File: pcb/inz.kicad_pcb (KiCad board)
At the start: 2 copper layers, 410 parts, among them U1 AMS1117-3.3, U2 ESP32-S3-WROOM-1

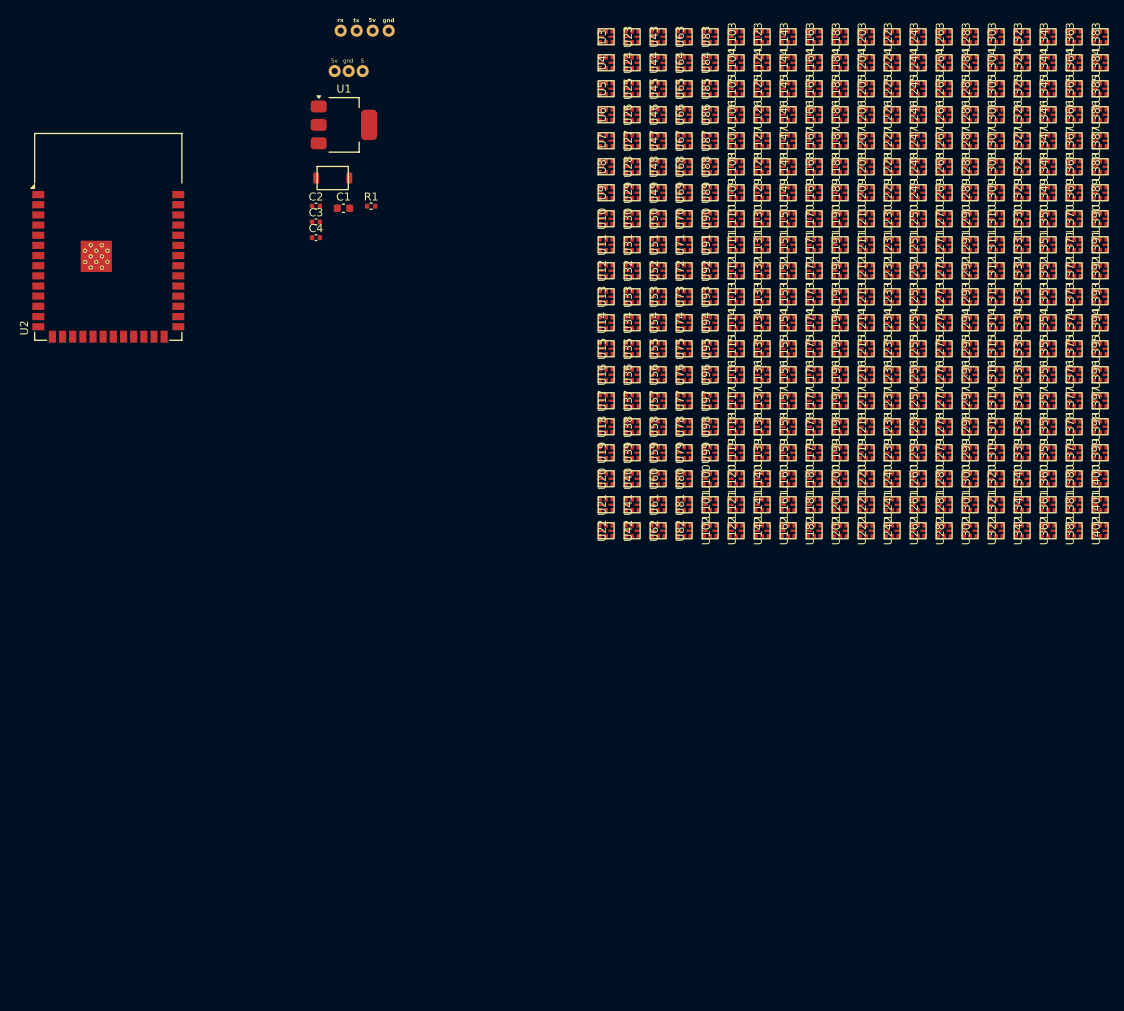
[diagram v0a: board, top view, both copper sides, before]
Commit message: pcb update
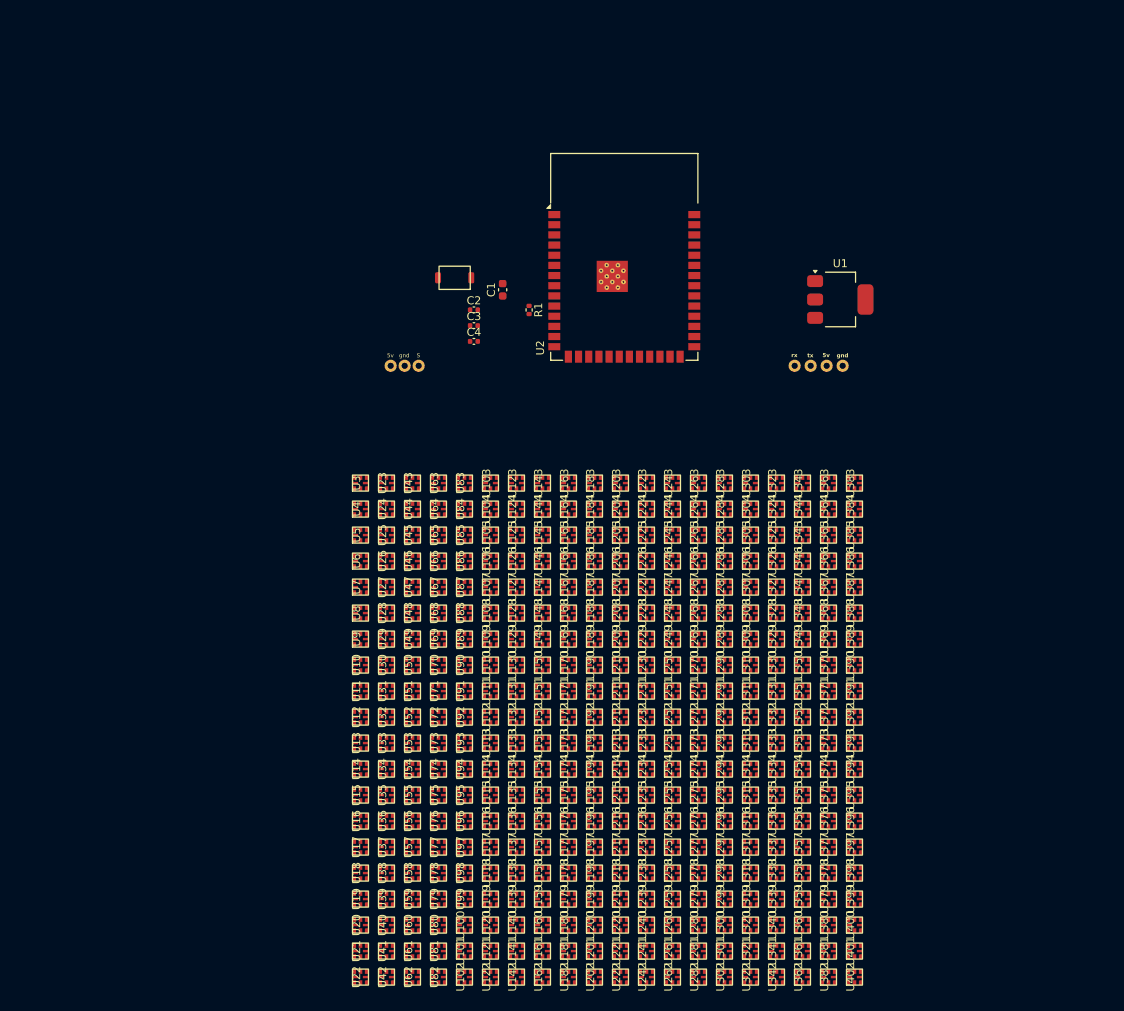
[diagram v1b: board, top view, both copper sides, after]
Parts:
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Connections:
- U103 pad 3: Net-(U103-CLI) -> Net-(U102-CLO)
- U103 pad 6: Net-(U103-DAI) -> Net-(U102-DAO)
- U104 pad 1: Net-(U103-CLI) -> Net-(U104-CLO)
- U104 pad 3: Net-(U104-CLI) -> Net-(U103-CLO)
- U104 pad 4: Net-(U103-DAI) -> Net-(U104-DAO)
- U104 pad 6: Net-(U104-DAI) -> Net-(U103-DAO)
- U105 pad 1: Net-(U104-CLI) -> Net-(U105-CLO)
- U105 pad 3: Net-(U105-CLI) -> Net-(U104-CLO)
- U105 pad 4: Net-(U104-DAI) -> Net-(U105-DAO)
- U105 pad 6: Net-(U105-DAI) -> Net-(U104-DAO)
- U106 pad 1: Net-(U105-CLI) -> Net-(U106-CLO)
- U106 pad 3: Net-(U106-CLI) -> Net-(U105-CLO)
- U106 pad 4: Net-(U105-DAI) -> Net-(U106-DAO)
- U106 pad 6: Net-(U106-DAI) -> Net-(U105-DAO)
- U107 pad 1: Net-(U106-CLI) -> Net-(U107-CLO)
- U107 pad 3: Net-(U107-CLI) -> Net-(U106-CLO)
- U107 pad 4: Net-(U106-DAI) -> Net-(U107-DAO)
- U107 pad 6: Net-(U107-DAI) -> Net-(U106-DAO)
- U108 pad 1: Net-(U107-CLI) -> Net-(U108-CLO)
- U108 pad 3: Net-(U108-CLI) -> Net-(U107-CLO)
- U108 pad 4: Net-(U107-DAI) -> Net-(U108-DAO)
- U108 pad 6: Net-(U108-DAI) -> Net-(U107-DAO)
- U109 pad 1: Net-(U108-CLI) -> Net-(U109-CLO)
- U109 pad 3: Net-(U109-CLI) -> Net-(U108-CLO)
- U109 pad 4: Net-(U108-DAI) -> Net-(U109-DAO)
- U109 pad 6: Net-(U109-DAI) -> Net-(U108-DAO)
- U110 pad 1: Net-(U109-CLI) -> Net-(U110-CLO)
- U110 pad 3: Net-(U110-CLI) -> Net-(U109-CLO)
- U110 pad 4: Net-(U109-DAI) -> Net-(U110-DAO)
- U110 pad 6: Net-(U110-DAI) -> Net-(U109-DAO)
- U111 pad 1: Net-(U110-CLI) -> Net-(U111-CLO)
- U111 pad 3: Net-(U111-CLI) -> Net-(U110-CLO)
- U111 pad 4: Net-(U110-DAI) -> Net-(U111-DAO)
- U111 pad 6: Net-(U111-DAI) -> Net-(U110-DAO)
- U112 pad 1: Net-(U111-CLI) -> Net-(U112-CLO)
- U112 pad 3: Net-(U112-CLI) -> Net-(U111-CLO)
- U112 pad 4: Net-(U111-DAI) -> Net-(U112-DAO)
- U112 pad 6: Net-(U112-DAI) -> Net-(U111-DAO)
- U113 pad 1: Net-(U112-CLI) -> Net-(U113-CLO)
- U113 pad 3: Net-(U113-CLI) -> Net-(U112-CLO)
- U113 pad 4: Net-(U112-DAI) -> Net-(U113-DAO)
- U113 pad 6: Net-(U113-DAI) -> Net-(U112-DAO)
- U114 pad 1: Net-(U113-CLI) -> Net-(U114-CLO)
- U114 pad 3: Net-(U114-CLI) -> Net-(U113-CLO)
- U114 pad 4: Net-(U113-DAI) -> Net-(U114-DAO)
- U114 pad 6: Net-(U114-DAI) -> Net-(U113-DAO)
- U115 pad 1: Net-(U114-CLI) -> Net-(U115-CLO)
- U115 pad 3: Net-(U115-CLI) -> Net-(U114-CLO)
- U115 pad 4: Net-(U114-DAI) -> Net-(U115-DAO)
- U115 pad 6: Net-(U115-DAI) -> Net-(U114-DAO)
- U116 pad 1: Net-(U115-CLI) -> Net-(U116-CLO)
- U116 pad 3: Net-(U116-CLI) -> Net-(U115-CLO)
- U116 pad 4: Net-(U115-DAI) -> Net-(U116-DAO)
- U116 pad 6: Net-(U116-DAI) -> Net-(U115-DAO)
- U117 pad 1: Net-(U116-CLI) -> Net-(U117-CLO)
- U117 pad 3: Net-(U117-CLI) -> Net-(U116-CLO)
- U117 pad 4: Net-(U116-DAI) -> Net-(U117-DAO)
- U117 pad 6: Net-(U117-DAI) -> Net-(U116-DAO)
- U118 pad 1: Net-(U117-CLI) -> Net-(U118-CLO)
- U118 pad 3: Net-(U118-CLI) -> Net-(U117-CLO)
- U118 pad 4: Net-(U117-DAI) -> Net-(U118-DAO)
- U118 pad 6: Net-(U118-DAI) -> Net-(U117-DAO)
- U119 pad 1: Net-(U118-CLI) -> Net-(U119-CLO)
- U119 pad 3: Net-(U119-CLI) -> Net-(U118-CLO)
- U119 pad 4: Net-(U118-DAI) -> Net-(U119-DAO)
- U119 pad 6: Net-(U119-DAI) -> Net-(U118-DAO)
- U120 pad 1: Net-(U119-CLI) -> Net-(U120-CLO)
- U120 pad 3: Net-(U120-CLI) -> Net-(U119-CLO)
- U120 pad 4: Net-(U119-DAI) -> Net-(U120-DAO)
- U120 pad 6: Net-(U120-DAI) -> Net-(U119-DAO)
- U121 pad 1: Net-(U120-CLI) -> Net-(U121-CLO)
- U121 pad 3: Net-(U121-CLI) -> Net-(U120-CLO)
- U121 pad 4: Net-(U120-DAI) -> Net-(U121-DAO)
- U121 pad 6: Net-(U121-DAI) -> Net-(U120-DAO)
- U122 pad 1: Net-(U121-CLI) -> Net-(U122-CLO)
- U122 pad 3: Net-(U102-CLO) -> Net-(U121-CLO)
- U122 pad 4: Net-(U121-DAI) -> Net-(U122-DAO)
- U122 pad 6: Net-(U102-DAO) -> Net-(U121-DAO)
- U123 pad 3: Net-(U103-CLO) -> Net-(U122-CLO)
- U123 pad 6: Net-(U103-DAO) -> Net-(U122-DAO)
- U143 pad 3: Net-(U143-CLI) -> Net-(U142-CLO)
- U143 pad 6: Net-(U143-DAI) -> Net-(U142-DAO)
- U144 pad 1: Net-(U143-CLI) -> Net-(U144-CLO)
- U144 pad 3: Net-(U144-CLI) -> Net-(U143-CLO)
- U144 pad 4: Net-(U143-DAI) -> Net-(U144-DAO)
- U144 pad 6: Net-(U144-DAI) -> Net-(U143-DAO)
- U145 pad 1: Net-(U144-CLI) -> Net-(U145-CLO)
- U145 pad 3: Net-(U145-CLI) -> Net-(U144-CLO)
- U145 pad 4: Net-(U144-DAI) -> Net-(U145-DAO)
- U145 pad 6: Net-(U145-DAI) -> Net-(U144-DAO)
- U146 pad 1: Net-(U145-CLI) -> Net-(U146-CLO)
- U146 pad 3: Net-(U146-CLI) -> Net-(U145-CLO)
- U146 pad 4: Net-(U145-DAI) -> Net-(U146-DAO)
- U146 pad 6: Net-(U146-DAI) -> Net-(U145-DAO)
- U147 pad 1: Net-(U146-CLI) -> Net-(U147-CLO)
- U147 pad 3: Net-(U147-CLI) -> Net-(U146-CLO)
- U147 pad 4: Net-(U146-DAI) -> Net-(U147-DAO)
- U147 pad 6: Net-(U147-DAI) -> Net-(U146-DAO)
- U148 pad 1: Net-(U147-CLI) -> Net-(U148-CLO)
- U148 pad 3: Net-(U148-CLI) -> Net-(U147-CLO)
- U148 pad 4: Net-(U147-DAI) -> Net-(U148-DAO)
- U148 pad 6: Net-(U148-DAI) -> Net-(U147-DAO)
- U149 pad 1: Net-(U148-CLI) -> Net-(U149-CLO)
- U149 pad 3: Net-(U149-CLI) -> Net-(U148-CLO)
- U149 pad 4: Net-(U148-DAI) -> Net-(U149-DAO)
- U149 pad 6: Net-(U149-DAI) -> Net-(U148-DAO)
- U150 pad 1: Net-(U149-CLI) -> Net-(U150-CLO)
- U150 pad 3: Net-(U150-CLI) -> Net-(U149-CLO)
- U150 pad 4: Net-(U149-DAI) -> Net-(U150-DAO)
- U150 pad 6: Net-(U150-DAI) -> Net-(U149-DAO)
- U151 pad 1: Net-(U150-CLI) -> Net-(U151-CLO)
- U151 pad 3: Net-(U151-CLI) -> Net-(U150-CLO)
- U151 pad 4: Net-(U150-DAI) -> Net-(U151-DAO)
- U151 pad 6: Net-(U151-DAI) -> Net-(U150-DAO)
- U152 pad 1: Net-(U151-CLI) -> Net-(U152-CLO)
- U152 pad 3: Net-(U152-CLI) -> Net-(U151-CLO)
- U152 pad 4: Net-(U151-DAI) -> Net-(U152-DAO)
- U152 pad 6: Net-(U152-DAI) -> Net-(U151-DAO)
- U153 pad 1: Net-(U152-CLI) -> Net-(U153-CLO)
- U153 pad 3: Net-(U153-CLI) -> Net-(U152-CLO)
- U153 pad 4: Net-(U152-DAI) -> Net-(U153-DAO)
- U153 pad 6: Net-(U153-DAI) -> Net-(U152-DAO)
- U154 pad 1: Net-(U153-CLI) -> Net-(U154-CLO)
- U154 pad 3: Net-(U154-CLI) -> Net-(U153-CLO)
- U154 pad 4: Net-(U153-DAI) -> Net-(U154-DAO)
- U154 pad 6: Net-(U154-DAI) -> Net-(U153-DAO)
- U155 pad 1: Net-(U154-CLI) -> Net-(U155-CLO)
- U155 pad 3: Net-(U155-CLI) -> Net-(U154-CLO)
- U155 pad 4: Net-(U154-DAI) -> Net-(U155-DAO)
- U155 pad 6: Net-(U155-DAI) -> Net-(U154-DAO)
- U156 pad 1: Net-(U155-CLI) -> Net-(U156-CLO)
- U156 pad 3: Net-(U156-CLI) -> Net-(U155-CLO)
- U156 pad 4: Net-(U155-DAI) -> Net-(U156-DAO)
- U156 pad 6: Net-(U156-DAI) -> Net-(U155-DAO)
- U157 pad 1: Net-(U156-CLI) -> Net-(U157-CLO)
- U157 pad 3: Net-(U157-CLI) -> Net-(U156-CLO)
- U157 pad 4: Net-(U156-DAI) -> Net-(U157-DAO)
- U157 pad 6: Net-(U157-DAI) -> Net-(U156-DAO)
- U158 pad 1: Net-(U157-CLI) -> Net-(U158-CLO)
- U158 pad 3: Net-(U158-CLI) -> Net-(U157-CLO)
- U158 pad 4: Net-(U157-DAI) -> Net-(U158-DAO)
- U158 pad 6: Net-(U158-DAI) -> Net-(U157-DAO)
- U159 pad 1: Net-(U158-CLI) -> Net-(U159-CLO)
- U159 pad 3: Net-(U159-CLI) -> Net-(U158-CLO)
- U159 pad 4: Net-(U158-DAI) -> Net-(U159-DAO)
- U159 pad 6: Net-(U159-DAI) -> Net-(U158-DAO)
- U160 pad 1: Net-(U159-CLI) -> Net-(U160-CLO)
- U160 pad 3: Net-(U160-CLI) -> Net-(U159-CLO)
- U160 pad 4: Net-(U159-DAI) -> Net-(U160-DAO)
- U160 pad 6: Net-(U160-DAI) -> Net-(U159-DAO)
- U161 pad 1: Net-(U160-CLI) -> Net-(U161-CLO)
- U161 pad 3: Net-(U161-CLI) -> Net-(U160-CLO)
- U161 pad 4: Net-(U160-DAI) -> Net-(U161-DAO)
- U161 pad 6: Net-(U161-DAI) -> Net-(U160-DAO)
- U162 pad 1: Net-(U161-CLI) -> Net-(U162-CLO)
- U162 pad 3: Net-(U142-CLO) -> Net-(U161-CLO)
- U162 pad 4: Net-(U161-DAI) -> Net-(U162-DAO)
- U162 pad 6: Net-(U142-DAO) -> Net-(U161-DAO)
- U163 pad 3: Net-(U143-CLO) -> Net-(U162-CLO)
- U163 pad 6: Net-(U143-DAO) -> Net-(U162-DAO)
- U183 pad 1: unconnected-(U183-CLO-Pad1) -> Net-(U183-CLO)
- U183 pad 3: Net-(U183-CLI) -> Net-(U182-CLO)
- U183 pad 4: unconnected-(U183-DAO-Pad4) -> Net-(U183-DAO)
- U183 pad 6: Net-(U183-DAI) -> Net-(U182-DAO)
- U184 pad 1: Net-(U183-CLI) -> Net-(U184-CLO)
- U184 pad 3: Net-(U184-CLI) -> Net-(U183-CLO)
- U184 pad 4: Net-(U183-DAI) -> Net-(U184-DAO)
- U184 pad 6: Net-(U184-DAI) -> Net-(U183-DAO)
- U185 pad 1: Net-(U184-CLI) -> Net-(U185-CLO)
- U185 pad 3: Net-(U185-CLI) -> Net-(U184-CLO)
- U185 pad 4: Net-(U184-DAI) -> Net-(U185-DAO)
- U185 pad 6: Net-(U185-DAI) -> Net-(U184-DAO)
- U186 pad 1: Net-(U185-CLI) -> Net-(U186-CLO)
- U186 pad 3: Net-(U186-CLI) -> Net-(U185-CLO)
- U186 pad 4: Net-(U185-DAI) -> Net-(U186-DAO)
- U186 pad 6: Net-(U186-DAI) -> Net-(U185-DAO)
- U187 pad 1: Net-(U186-CLI) -> Net-(U187-CLO)
- U187 pad 3: Net-(U187-CLI) -> Net-(U186-CLO)
- U187 pad 4: Net-(U186-DAI) -> Net-(U187-DAO)
- U187 pad 6: Net-(U187-DAI) -> Net-(U186-DAO)
- U188 pad 1: Net-(U187-CLI) -> Net-(U188-CLO)
- U188 pad 3: Net-(U188-CLI) -> Net-(U187-CLO)
- U188 pad 4: Net-(U187-DAI) -> Net-(U188-DAO)
- U188 pad 6: Net-(U188-DAI) -> Net-(U187-DAO)
- U189 pad 1: Net-(U188-CLI) -> Net-(U189-CLO)
- U189 pad 3: Net-(U189-CLI) -> Net-(U188-CLO)
- U189 pad 4: Net-(U188-DAI) -> Net-(U189-DAO)
- U189 pad 6: Net-(U189-DAI) -> Net-(U188-DAO)
- U190 pad 1: Net-(U189-CLI) -> Net-(U190-CLO)
- U190 pad 3: Net-(U190-CLI) -> Net-(U189-CLO)
- U190 pad 4: Net-(U189-DAI) -> Net-(U190-DAO)
- U190 pad 6: Net-(U190-DAI) -> Net-(U189-DAO)
- U191 pad 1: Net-(U190-CLI) -> Net-(U191-CLO)
- U191 pad 3: Net-(U191-CLI) -> Net-(U190-CLO)
- U191 pad 4: Net-(U190-DAI) -> Net-(U191-DAO)
- U191 pad 6: Net-(U191-DAI) -> Net-(U190-DAO)
- U192 pad 1: Net-(U191-CLI) -> Net-(U192-CLO)
- U192 pad 3: Net-(U192-CLI) -> Net-(U191-CLO)
- U192 pad 4: Net-(U191-DAI) -> Net-(U192-DAO)
- U192 pad 6: Net-(U192-DAI) -> Net-(U191-DAO)
- U193 pad 1: Net-(U192-CLI) -> Net-(U193-CLO)
- U193 pad 3: Net-(U193-CLI) -> Net-(U192-CLO)
- U193 pad 4: Net-(U192-DAI) -> Net-(U193-DAO)
- U193 pad 6: Net-(U193-DAI) -> Net-(U192-DAO)
- U194 pad 1: Net-(U193-CLI) -> Net-(U194-CLO)
- U194 pad 3: Net-(U194-CLI) -> Net-(U193-CLO)
- U194 pad 4: Net-(U193-DAI) -> Net-(U194-DAO)
- U194 pad 6: Net-(U194-DAI) -> Net-(U193-DAO)
- U195 pad 1: Net-(U194-CLI) -> Net-(U195-CLO)
- U195 pad 3: Net-(U195-CLI) -> Net-(U194-CLO)
- U195 pad 4: Net-(U194-DAI) -> Net-(U195-DAO)
- U195 pad 6: Net-(U195-DAI) -> Net-(U194-DAO)
- U196 pad 1: Net-(U195-CLI) -> Net-(U196-CLO)
- U196 pad 3: Net-(U196-CLI) -> Net-(U195-CLO)
- U196 pad 4: Net-(U195-DAI) -> Net-(U196-DAO)
- U196 pad 6: Net-(U196-DAI) -> Net-(U195-DAO)
- U197 pad 1: Net-(U196-CLI) -> Net-(U197-CLO)
- U197 pad 3: Net-(U197-CLI) -> Net-(U196-CLO)
- U197 pad 4: Net-(U196-DAI) -> Net-(U197-DAO)
- U197 pad 6: Net-(U197-DAI) -> Net-(U196-DAO)
- U198 pad 1: Net-(U197-CLI) -> Net-(U198-CLO)
- U198 pad 3: Net-(U198-CLI) -> Net-(U197-CLO)
- U198 pad 4: Net-(U197-DAI) -> Net-(U198-DAO)
- U198 pad 6: Net-(U198-DAI) -> Net-(U197-DAO)
- U199 pad 1: Net-(U198-CLI) -> Net-(U199-CLO)
- U199 pad 3: Net-(U199-CLI) -> Net-(U198-CLO)
- U199 pad 4: Net-(U198-DAI) -> Net-(U199-DAO)
- U199 pad 6: Net-(U199-DAI) -> Net-(U198-DAO)
- U200 pad 1: Net-(U199-CLI) -> Net-(U200-CLO)
- U200 pad 3: Net-(U200-CLI) -> Net-(U199-CLO)
- U200 pad 4: Net-(U199-DAI) -> Net-(U200-DAO)
- U200 pad 6: Net-(U200-DAI) -> Net-(U199-DAO)
- U201 pad 1: Net-(U200-CLI) -> Net-(U201-CLO)
- U201 pad 3: Net-(U201-CLI) -> Net-(U200-CLO)
- U201 pad 4: Net-(U200-DAI) -> Net-(U201-DAO)
- U201 pad 6: Net-(U201-DAI) -> Net-(U200-DAO)
- U202 pad 1: Net-(U201-CLI) -> unconnected-(U202-CLO-Pad1)
- U202 pad 3: Net-(U182-CLO) -> Net-(U201-CLO)
- U202 pad 4: Net-(U201-DAI) -> unconnected-(U202-DAO-Pad4)
- U202 pad 6: Net-(U182-DAO) -> Net-(U201-DAO)
- U223 pad 3: Net-(U223-CLI) -> Net-(U222-CLO)
- U223 pad 6: Net-(U223-DAI) -> Net-(U222-DAO)
- U224 pad 1: Net-(U223-CLI) -> Net-(U224-CLO)
- U224 pad 3: Net-(U224-CLI) -> Net-(U223-CLO)
- U224 pad 4: Net-(U223-DAI) -> Net-(U224-DAO)
- U224 pad 6: Net-(U224-DAI) -> Net-(U223-DAO)
- U225 pad 1: Net-(U224-CLI) -> Net-(U225-CLO)
- U225 pad 3: Net-(U225-CLI) -> Net-(U224-CLO)
- U225 pad 4: Net-(U224-DAI) -> Net-(U225-DAO)
- U225 pad 6: Net-(U225-DAI) -> Net-(U224-DAO)
- U226 pad 1: Net-(U225-CLI) -> Net-(U226-CLO)
- U226 pad 3: Net-(U226-CLI) -> Net-(U225-CLO)
- U226 pad 4: Net-(U225-DAI) -> Net-(U226-DAO)
- U226 pad 6: Net-(U226-DAI) -> Net-(U225-DAO)
- U227 pad 1: Net-(U226-CLI) -> Net-(U227-CLO)
- U227 pad 3: Net-(U227-CLI) -> Net-(U226-CLO)
- U227 pad 4: Net-(U226-DAI) -> Net-(U227-DAO)
- U227 pad 6: Net-(U227-DAI) -> Net-(U226-DAO)
- U228 pad 1: Net-(U227-CLI) -> Net-(U228-CLO)
- U228 pad 3: Net-(U228-CLI) -> Net-(U227-CLO)
- U228 pad 4: Net-(U227-DAI) -> Net-(U228-DAO)
- U228 pad 6: Net-(U228-DAI) -> Net-(U227-DAO)
- U229 pad 1: Net-(U228-CLI) -> Net-(U229-CLO)
- U229 pad 3: Net-(U229-CLI) -> Net-(U228-CLO)
- U229 pad 4: Net-(U228-DAI) -> Net-(U229-DAO)
- U229 pad 6: Net-(U229-DAI) -> Net-(U228-DAO)
- U23 pad 3: Net-(U23-CLI) -> Net-(U22-CLO)
- U23 pad 6: Net-(U23-DAI) -> Net-(U22-DAO)
- U230 pad 1: Net-(U229-CLI) -> Net-(U230-CLO)
- U230 pad 3: Net-(U230-CLI) -> Net-(U229-CLO)
- U230 pad 4: Net-(U229-DAI) -> Net-(U230-DAO)
- U230 pad 6: Net-(U230-DAI) -> Net-(U229-DAO)
- U231 pad 1: Net-(U230-CLI) -> Net-(U231-CLO)
- U231 pad 3: Net-(U231-CLI) -> Net-(U230-CLO)
- U231 pad 4: Net-(U230-DAI) -> Net-(U231-DAO)
- U231 pad 6: Net-(U231-DAI) -> Net-(U230-DAO)
- U232 pad 1: Net-(U231-CLI) -> Net-(U232-CLO)
- U232 pad 3: Net-(U232-CLI) -> Net-(U231-CLO)
- U232 pad 4: Net-(U231-DAI) -> Net-(U232-DAO)
- U232 pad 6: Net-(U232-DAI) -> Net-(U231-DAO)
- U233 pad 1: Net-(U232-CLI) -> Net-(U233-CLO)
- U233 pad 3: Net-(U233-CLI) -> Net-(U232-CLO)
- U233 pad 4: Net-(U232-DAI) -> Net-(U233-DAO)
- U233 pad 6: Net-(U233-DAI) -> Net-(U232-DAO)
- U234 pad 1: Net-(U233-CLI) -> Net-(U234-CLO)
- U234 pad 3: Net-(U234-CLI) -> Net-(U233-CLO)
- U234 pad 4: Net-(U233-DAI) -> Net-(U234-DAO)
- U234 pad 6: Net-(U234-DAI) -> Net-(U233-DAO)
- U235 pad 1: Net-(U234-CLI) -> Net-(U235-CLO)
- U235 pad 3: Net-(U235-CLI) -> Net-(U234-CLO)
- U235 pad 4: Net-(U234-DAI) -> Net-(U235-DAO)
- U235 pad 6: Net-(U235-DAI) -> Net-(U234-DAO)
- U236 pad 1: Net-(U235-CLI) -> Net-(U236-CLO)
- U236 pad 3: Net-(U236-CLI) -> Net-(U235-CLO)
- U236 pad 4: Net-(U235-DAI) -> Net-(U236-DAO)
- U236 pad 6: Net-(U236-DAI) -> Net-(U235-DAO)
- U237 pad 1: Net-(U236-CLI) -> Net-(U237-CLO)
- U237 pad 3: Net-(U237-CLI) -> Net-(U236-CLO)
- U237 pad 4: Net-(U236-DAI) -> Net-(U237-DAO)
- U237 pad 6: Net-(U237-DAI) -> Net-(U236-DAO)
- U238 pad 1: Net-(U237-CLI) -> Net-(U238-CLO)
- U238 pad 3: Net-(U238-CLI) -> Net-(U237-CLO)
- U238 pad 4: Net-(U237-DAI) -> Net-(U238-DAO)
- U238 pad 6: Net-(U238-DAI) -> Net-(U237-DAO)
- U239 pad 1: Net-(U238-CLI) -> Net-(U239-CLO)
- U239 pad 3: Net-(U239-CLI) -> Net-(U238-CLO)
- U239 pad 4: Net-(U238-DAI) -> Net-(U239-DAO)
- U239 pad 6: Net-(U239-DAI) -> Net-(U238-DAO)
- U24 pad 1: Net-(U23-CLI) -> Net-(U24-CLO)
- U24 pad 3: Net-(U24-CLI) -> Net-(U23-CLO)
- U24 pad 4: Net-(U23-DAI) -> Net-(U24-DAO)
- U24 pad 6: Net-(U24-DAI) -> Net-(U23-DAO)
- U240 pad 1: Net-(U239-CLI) -> Net-(U240-CLO)
- U240 pad 3: Net-(U240-CLI) -> Net-(U239-CLO)
- U240 pad 4: Net-(U239-DAI) -> Net-(U240-DAO)
- U240 pad 6: Net-(U240-DAI) -> Net-(U239-DAO)
- U241 pad 1: Net-(U240-CLI) -> Net-(U241-CLO)
- U241 pad 3: Net-(U241-CLI) -> Net-(U240-CLO)
- U241 pad 4: Net-(U240-DAI) -> Net-(U241-DAO)
- U241 pad 6: Net-(U241-DAI) -> Net-(U240-DAO)
- U242 pad 1: Net-(U241-CLI) -> Net-(U242-CLO)
- U242 pad 3: Net-(U222-CLO) -> Net-(U241-CLO)
- U242 pad 4: Net-(U241-DAI) -> Net-(U242-DAO)
- U242 pad 6: Net-(U222-DAO) -> Net-(U241-DAO)
- U243 pad 3: Net-(U223-CLO) -> Net-(U242-CLO)
- U243 pad 6: Net-(U223-DAO) -> Net-(U242-DAO)
- U25 pad 1: Net-(U24-CLI) -> Net-(U25-CLO)
- U25 pad 3: Net-(U25-CLI) -> Net-(U24-CLO)
- U25 pad 4: Net-(U24-DAI) -> Net-(U25-DAO)
- U25 pad 6: Net-(U25-DAI) -> Net-(U24-DAO)
- U26 pad 1: Net-(U25-CLI) -> Net-(U26-CLO)
- U26 pad 3: Net-(U26-CLI) -> Net-(U25-CLO)
- U26 pad 4: Net-(U25-DAI) -> Net-(U26-DAO)
- U26 pad 6: Net-(U26-DAI) -> Net-(U25-DAO)
- U263 pad 3: Net-(U263-CLI) -> Net-(U262-CLO)
- U263 pad 6: Net-(U263-DAI) -> Net-(U262-DAO)
- U264 pad 1: Net-(U263-CLI) -> Net-(U264-CLO)
- U264 pad 3: Net-(U264-CLI) -> Net-(U263-CLO)
- U264 pad 4: Net-(U263-DAI) -> Net-(U264-DAO)
- U264 pad 6: Net-(U264-DAI) -> Net-(U263-DAO)
- U265 pad 1: Net-(U264-CLI) -> Net-(U265-CLO)
- U265 pad 3: Net-(U265-CLI) -> Net-(U264-CLO)
- U265 pad 4: Net-(U264-DAI) -> Net-(U265-DAO)
- U265 pad 6: Net-(U265-DAI) -> Net-(U264-DAO)
- U266 pad 1: Net-(U265-CLI) -> Net-(U266-CLO)
- U266 pad 3: Net-(U266-CLI) -> Net-(U265-CLO)
- U266 pad 4: Net-(U265-DAI) -> Net-(U266-DAO)
- U266 pad 6: Net-(U266-DAI) -> Net-(U265-DAO)
- U267 pad 1: Net-(U266-CLI) -> Net-(U267-CLO)
- U267 pad 3: Net-(U267-CLI) -> Net-(U266-CLO)
- U267 pad 4: Net-(U266-DAI) -> Net-(U267-DAO)
- U267 pad 6: Net-(U267-DAI) -> Net-(U266-DAO)
- U268 pad 1: Net-(U267-CLI) -> Net-(U268-CLO)
- U268 pad 3: Net-(U268-CLI) -> Net-(U267-CLO)
- U268 pad 4: Net-(U267-DAI) -> Net-(U268-DAO)
- U268 pad 6: Net-(U268-DAI) -> Net-(U267-DAO)
- U269 pad 1: Net-(U268-CLI) -> Net-(U269-CLO)
- U269 pad 3: Net-(U269-CLI) -> Net-(U268-CLO)
- U269 pad 4: Net-(U268-DAI) -> Net-(U269-DAO)
- U269 pad 6: Net-(U269-DAI) -> Net-(U268-DAO)
- U27 pad 1: Net-(U26-CLI) -> Net-(U27-CLO)
- U27 pad 3: Net-(U27-CLI) -> Net-(U26-CLO)
- U27 pad 4: Net-(U26-DAI) -> Net-(U27-DAO)
- U27 pad 6: Net-(U27-DAI) -> Net-(U26-DAO)
- U270 pad 1: Net-(U269-CLI) -> Net-(U270-CLO)
- U270 pad 3: Net-(U270-CLI) -> Net-(U269-CLO)
- U270 pad 4: Net-(U269-DAI) -> Net-(U270-DAO)
- U270 pad 6: Net-(U270-DAI) -> Net-(U269-DAO)
- U271 pad 1: Net-(U270-CLI) -> Net-(U271-CLO)
- U271 pad 3: Net-(U271-CLI) -> Net-(U270-CLO)
- U271 pad 4: Net-(U270-DAI) -> Net-(U271-DAO)
- U271 pad 6: Net-(U271-DAI) -> Net-(U270-DAO)
- U272 pad 1: Net-(U271-CLI) -> Net-(U272-CLO)
- U272 pad 3: Net-(U272-CLI) -> Net-(U271-CLO)
- U272 pad 4: Net-(U271-DAI) -> Net-(U272-DAO)
- U272 pad 6: Net-(U272-DAI) -> Net-(U271-DAO)
- U273 pad 1: Net-(U272-CLI) -> Net-(U273-CLO)
- U273 pad 3: Net-(U273-CLI) -> Net-(U272-CLO)
- U273 pad 4: Net-(U272-DAI) -> Net-(U273-DAO)
- U273 pad 6: Net-(U273-DAI) -> Net-(U272-DAO)
- U274 pad 1: Net-(U273-CLI) -> Net-(U274-CLO)
- U274 pad 3: Net-(U274-CLI) -> Net-(U273-CLO)
- U274 pad 4: Net-(U273-DAI) -> Net-(U274-DAO)
- U274 pad 6: Net-(U274-DAI) -> Net-(U273-DAO)
- U275 pad 1: Net-(U274-CLI) -> Net-(U275-CLO)
- U275 pad 3: Net-(U275-CLI) -> Net-(U274-CLO)
- U275 pad 4: Net-(U274-DAI) -> Net-(U275-DAO)
- U275 pad 6: Net-(U275-DAI) -> Net-(U274-DAO)
- U276 pad 1: Net-(U275-CLI) -> Net-(U276-CLO)
- U276 pad 3: Net-(U276-CLI) -> Net-(U275-CLO)
- U276 pad 4: Net-(U275-DAI) -> Net-(U276-DAO)
- U276 pad 6: Net-(U276-DAI) -> Net-(U275-DAO)
- U277 pad 1: Net-(U276-CLI) -> Net-(U277-CLO)
- U277 pad 3: Net-(U277-CLI) -> Net-(U276-CLO)
- U277 pad 4: Net-(U276-DAI) -> Net-(U277-DAO)
- U277 pad 6: Net-(U277-DAI) -> Net-(U276-DAO)
- U278 pad 1: Net-(U277-CLI) -> Net-(U278-CLO)
- U278 pad 3: Net-(U278-CLI) -> Net-(U277-CLO)
- U278 pad 4: Net-(U277-DAI) -> Net-(U278-DAO)
- U278 pad 6: Net-(U278-DAI) -> Net-(U277-DAO)
- U279 pad 1: Net-(U278-CLI) -> Net-(U279-CLO)
- U279 pad 3: Net-(U279-CLI) -> Net-(U278-CLO)
- U279 pad 4: Net-(U278-DAI) -> Net-(U279-DAO)
- U279 pad 6: Net-(U279-DAI) -> Net-(U278-DAO)
- U28 pad 1: Net-(U27-CLI) -> Net-(U28-CLO)
- U28 pad 3: Net-(U28-CLI) -> Net-(U27-CLO)
- U28 pad 4: Net-(U27-DAI) -> Net-(U28-DAO)
- U28 pad 6: Net-(U28-DAI) -> Net-(U27-DAO)
- U280 pad 1: Net-(U279-CLI) -> Net-(U280-CLO)
- U280 pad 3: Net-(U280-CLI) -> Net-(U279-CLO)
- U280 pad 4: Net-(U279-DAI) -> Net-(U280-DAO)
- U280 pad 6: Net-(U280-DAI) -> Net-(U279-DAO)
- U281 pad 1: Net-(U280-CLI) -> Net-(U281-CLO)
- U281 pad 3: Net-(U281-CLI) -> Net-(U280-CLO)
- U281 pad 4: Net-(U280-DAI) -> Net-(U281-DAO)
- U281 pad 6: Net-(U281-DAI) -> Net-(U280-DAO)
- U282 pad 1: Net-(U281-CLI) -> Net-(U282-CLO)
- U282 pad 3: Net-(U262-CLO) -> Net-(U281-CLO)
- U282 pad 4: Net-(U281-DAI) -> Net-(U282-DAO)
- U282 pad 6: Net-(U262-DAO) -> Net-(U281-DAO)
- U283 pad 3: Net-(U263-CLO) -> Net-(U282-CLO)
- U283 pad 6: Net-(U263-DAO) -> Net-(U282-DAO)
- U29 pad 1: Net-(U28-CLI) -> Net-(U29-CLO)
- U29 pad 3: Net-(U29-CLI) -> Net-(U28-CLO)
- U29 pad 4: Net-(U28-DAI) -> Net-(U29-DAO)
- U29 pad 6: Net-(U29-DAI) -> Net-(U28-DAO)
- U30 pad 1: Net-(U29-CLI) -> Net-(U30-CLO)
- U30 pad 3: Net-(U30-CLI) -> Net-(U29-CLO)
- U30 pad 4: Net-(U29-DAI) -> Net-(U30-DAO)
- U30 pad 6: Net-(U30-DAI) -> Net-(U29-DAO)
- U303 pad 3: Net-(U303-CLI) -> Net-(U302-CLO)
- U303 pad 6: Net-(U303-DAI) -> Net-(U302-DAO)
- U304 pad 1: Net-(U303-CLI) -> Net-(U304-CLO)
- U304 pad 3: Net-(U304-CLI) -> Net-(U303-CLO)
- U304 pad 4: Net-(U303-DAI) -> Net-(U304-DAO)
- U304 pad 6: Net-(U304-DAI) -> Net-(U303-DAO)
- U305 pad 1: Net-(U304-CLI) -> Net-(U305-CLO)
- U305 pad 3: Net-(U305-CLI) -> Net-(U304-CLO)
- U305 pad 4: Net-(U304-DAI) -> Net-(U305-DAO)
- U305 pad 6: Net-(U305-DAI) -> Net-(U304-DAO)
- U306 pad 1: Net-(U305-CLI) -> Net-(U306-CLO)
- U306 pad 3: Net-(U306-CLI) -> Net-(U305-CLO)
- U306 pad 4: Net-(U305-DAI) -> Net-(U306-DAO)
- U306 pad 6: Net-(U306-DAI) -> Net-(U305-DAO)
- U307 pad 1: Net-(U306-CLI) -> Net-(U307-CLO)
- U307 pad 3: Net-(U307-CLI) -> Net-(U306-CLO)
- U307 pad 4: Net-(U306-DAI) -> Net-(U307-DAO)
- U307 pad 6: Net-(U307-DAI) -> Net-(U306-DAO)
- U308 pad 1: Net-(U307-CLI) -> Net-(U308-CLO)
- U308 pad 3: Net-(U308-CLI) -> Net-(U307-CLO)
- U308 pad 4: Net-(U307-DAI) -> Net-(U308-DAO)
- U308 pad 6: Net-(U308-DAI) -> Net-(U307-DAO)
- U309 pad 1: Net-(U308-CLI) -> Net-(U309-CLO)
- U309 pad 3: Net-(U309-CLI) -> Net-(U308-CLO)
- U309 pad 4: Net-(U308-DAI) -> Net-(U309-DAO)
- U309 pad 6: Net-(U309-DAI) -> Net-(U308-DAO)
- U31 pad 1: Net-(U30-CLI) -> Net-(U31-CLO)
- U31 pad 3: Net-(U31-CLI) -> Net-(U30-CLO)
- U31 pad 4: Net-(U30-DAI) -> Net-(U31-DAO)
- U31 pad 6: Net-(U31-DAI) -> Net-(U30-DAO)
- U310 pad 1: Net-(U309-CLI) -> Net-(U310-CLO)
- U310 pad 3: Net-(U310-CLI) -> Net-(U309-CLO)
- U310 pad 4: Net-(U309-DAI) -> Net-(U310-DAO)
- U310 pad 6: Net-(U310-DAI) -> Net-(U309-DAO)
- U311 pad 1: Net-(U310-CLI) -> Net-(U311-CLO)
- U311 pad 3: Net-(U311-CLI) -> Net-(U310-CLO)
- U311 pad 4: Net-(U310-DAI) -> Net-(U311-DAO)
- U311 pad 6: Net-(U311-DAI) -> Net-(U310-DAO)
- U312 pad 1: Net-(U311-CLI) -> Net-(U312-CLO)
- U312 pad 3: Net-(U312-CLI) -> Net-(U311-CLO)
- U312 pad 4: Net-(U311-DAI) -> Net-(U312-DAO)
- U312 pad 6: Net-(U312-DAI) -> Net-(U311-DAO)
- U313 pad 1: Net-(U312-CLI) -> Net-(U313-CLO)
- U313 pad 3: Net-(U313-CLI) -> Net-(U312-CLO)
- U313 pad 4: Net-(U312-DAI) -> Net-(U313-DAO)
- U313 pad 6: Net-(U313-DAI) -> Net-(U312-DAO)
- U314 pad 1: Net-(U313-CLI) -> Net-(U314-CLO)
- U314 pad 3: Net-(U314-CLI) -> Net-(U313-CLO)
- U314 pad 4: Net-(U313-DAI) -> Net-(U314-DAO)
- U314 pad 6: Net-(U314-DAI) -> Net-(U313-DAO)
- U315 pad 1: Net-(U314-CLI) -> Net-(U315-CLO)
- U315 pad 3: Net-(U315-CLI) -> Net-(U314-CLO)
- U315 pad 4: Net-(U314-DAI) -> Net-(U315-DAO)
- U315 pad 6: Net-(U315-DAI) -> Net-(U314-DAO)
- U316 pad 1: Net-(U315-CLI) -> Net-(U316-CLO)
- U316 pad 3: Net-(U316-CLI) -> Net-(U315-CLO)
- U316 pad 4: Net-(U315-DAI) -> Net-(U316-DAO)
- U316 pad 6: Net-(U316-DAI) -> Net-(U315-DAO)
- U317 pad 1: Net-(U316-CLI) -> Net-(U317-CLO)
- U317 pad 3: Net-(U317-CLI) -> Net-(U316-CLO)
- U317 pad 4: Net-(U316-DAI) -> Net-(U317-DAO)
- U317 pad 6: Net-(U317-DAI) -> Net-(U316-DAO)
- U318 pad 1: Net-(U317-CLI) -> Net-(U318-CLO)
- U318 pad 3: Net-(U318-CLI) -> Net-(U317-CLO)
- U318 pad 4: Net-(U317-DAI) -> Net-(U318-DAO)
- U318 pad 6: Net-(U318-DAI) -> Net-(U317-DAO)
- U319 pad 1: Net-(U318-CLI) -> Net-(U319-CLO)
- U319 pad 3: Net-(U319-CLI) -> Net-(U318-CLO)
- U319 pad 4: Net-(U318-DAI) -> Net-(U319-DAO)
- U319 pad 6: Net-(U319-DAI) -> Net-(U318-DAO)
- U32 pad 1: Net-(U31-CLI) -> Net-(U32-CLO)
- U32 pad 3: Net-(U32-CLI) -> Net-(U31-CLO)
- U32 pad 4: Net-(U31-DAI) -> Net-(U32-DAO)
- U32 pad 6: Net-(U32-DAI) -> Net-(U31-DAO)
- U320 pad 1: Net-(U319-CLI) -> Net-(U320-CLO)
- U320 pad 3: Net-(U320-CLI) -> Net-(U319-CLO)
- U320 pad 4: Net-(U319-DAI) -> Net-(U320-DAO)
- U320 pad 6: Net-(U320-DAI) -> Net-(U319-DAO)
- U321 pad 1: Net-(U320-CLI) -> Net-(U321-CLO)
- U321 pad 3: Net-(U321-CLI) -> Net-(U320-CLO)
- U321 pad 4: Net-(U320-DAI) -> Net-(U321-DAO)
- U321 pad 6: Net-(U321-DAI) -> Net-(U320-DAO)
- U322 pad 1: Net-(U321-CLI) -> Net-(U322-CLO)
- U322 pad 3: Net-(U302-CLO) -> Net-(U321-CLO)
- U322 pad 4: Net-(U321-DAI) -> Net-(U322-DAO)
- U322 pad 6: Net-(U302-DAO) -> Net-(U321-DAO)
- U323 pad 3: Net-(U303-CLO) -> Net-(U322-CLO)
- U323 pad 6: Net-(U303-DAO) -> Net-(U322-DAO)
- U33 pad 1: Net-(U32-CLI) -> Net-(U33-CLO)
- U33 pad 3: Net-(U33-CLI) -> Net-(U32-CLO)
- U33 pad 4: Net-(U32-DAI) -> Net-(U33-DAO)
- U33 pad 6: Net-(U33-DAI) -> Net-(U32-DAO)
- U34 pad 1: Net-(U33-CLI) -> Net-(U34-CLO)
- U34 pad 3: Net-(U34-CLI) -> Net-(U33-CLO)
- U34 pad 4: Net-(U33-DAI) -> Net-(U34-DAO)
- U34 pad 6: Net-(U34-DAI) -> Net-(U33-DAO)
- U343 pad 3: Net-(U343-CLI) -> Net-(U342-CLO)
- U343 pad 6: Net-(U343-DAI) -> Net-(U342-DAO)
- U344 pad 1: Net-(U343-CLI) -> Net-(U344-CLO)
- U344 pad 3: Net-(U344-CLI) -> Net-(U343-CLO)
- U344 pad 4: Net-(U343-DAI) -> Net-(U344-DAO)
- U344 pad 6: Net-(U344-DAI) -> Net-(U343-DAO)
- U345 pad 1: Net-(U344-CLI) -> Net-(U345-CLO)
- U345 pad 3: Net-(U345-CLI) -> Net-(U344-CLO)
- U345 pad 4: Net-(U344-DAI) -> Net-(U345-DAO)
- U345 pad 6: Net-(U345-DAI) -> Net-(U344-DAO)
- U346 pad 1: Net-(U345-CLI) -> Net-(U346-CLO)
- U346 pad 3: Net-(U346-CLI) -> Net-(U345-CLO)
- U346 pad 4: Net-(U345-DAI) -> Net-(U346-DAO)
- U346 pad 6: Net-(U346-DAI) -> Net-(U345-DAO)
- U347 pad 1: Net-(U346-CLI) -> Net-(U347-CLO)
- U347 pad 3: Net-(U347-CLI) -> Net-(U346-CLO)
- U347 pad 4: Net-(U346-DAI) -> Net-(U347-DAO)
- U347 pad 6: Net-(U347-DAI) -> Net-(U346-DAO)
- U348 pad 1: Net-(U347-CLI) -> Net-(U348-CLO)
- U348 pad 3: Net-(U348-CLI) -> Net-(U347-CLO)
- U348 pad 4: Net-(U347-DAI) -> Net-(U348-DAO)
- U348 pad 6: Net-(U348-DAI) -> Net-(U347-DAO)
- U349 pad 1: Net-(U348-CLI) -> Net-(U349-CLO)
- U349 pad 3: Net-(U349-CLI) -> Net-(U348-CLO)
- U349 pad 4: Net-(U348-DAI) -> Net-(U349-DAO)
- U349 pad 6: Net-(U349-DAI) -> Net-(U348-DAO)
- U35 pad 1: Net-(U34-CLI) -> Net-(U35-CLO)
- U35 pad 3: Net-(U35-CLI) -> Net-(U34-CLO)
- U35 pad 4: Net-(U34-DAI) -> Net-(U35-DAO)
- U35 pad 6: Net-(U35-DAI) -> Net-(U34-DAO)
- U350 pad 1: Net-(U349-CLI) -> Net-(U350-CLO)
- U350 pad 3: Net-(U350-CLI) -> Net-(U349-CLO)
- U350 pad 4: Net-(U349-DAI) -> Net-(U350-DAO)
- U350 pad 6: Net-(U350-DAI) -> Net-(U349-DAO)
- U351 pad 1: Net-(U350-CLI) -> Net-(U351-CLO)
- U351 pad 3: Net-(U351-CLI) -> Net-(U350-CLO)
- U351 pad 4: Net-(U350-DAI) -> Net-(U351-DAO)
- U351 pad 6: Net-(U351-DAI) -> Net-(U350-DAO)
- U352 pad 1: Net-(U351-CLI) -> Net-(U352-CLO)
- U352 pad 3: Net-(U352-CLI) -> Net-(U351-CLO)
- U352 pad 4: Net-(U351-DAI) -> Net-(U352-DAO)
- U352 pad 6: Net-(U352-DAI) -> Net-(U351-DAO)
- U353 pad 1: Net-(U352-CLI) -> Net-(U353-CLO)
- U353 pad 3: Net-(U353-CLI) -> Net-(U352-CLO)
- U353 pad 4: Net-(U352-DAI) -> Net-(U353-DAO)
- U353 pad 6: Net-(U353-DAI) -> Net-(U352-DAO)
- U354 pad 1: Net-(U353-CLI) -> Net-(U354-CLO)
- U354 pad 3: Net-(U354-CLI) -> Net-(U353-CLO)
- U354 pad 4: Net-(U353-DAI) -> Net-(U354-DAO)
- U354 pad 6: Net-(U354-DAI) -> Net-(U353-DAO)
- U355 pad 1: Net-(U354-CLI) -> Net-(U355-CLO)
- U355 pad 3: Net-(U355-CLI) -> Net-(U354-CLO)
- U355 pad 4: Net-(U354-DAI) -> Net-(U355-DAO)
- U355 pad 6: Net-(U355-DAI) -> Net-(U354-DAO)
- U356 pad 1: Net-(U355-CLI) -> Net-(U356-CLO)
- U356 pad 3: Net-(U356-CLI) -> Net-(U355-CLO)
- U356 pad 4: Net-(U355-DAI) -> Net-(U356-DAO)
- U356 pad 6: Net-(U356-DAI) -> Net-(U355-DAO)
- U357 pad 1: Net-(U356-CLI) -> Net-(U357-CLO)
- U357 pad 3: Net-(U357-CLI) -> Net-(U356-CLO)
- U357 pad 4: Net-(U356-DAI) -> Net-(U357-DAO)
- U357 pad 6: Net-(U357-DAI) -> Net-(U356-DAO)
- U358 pad 1: Net-(U357-CLI) -> Net-(U358-CLO)
- U358 pad 3: Net-(U358-CLI) -> Net-(U357-CLO)
- U358 pad 4: Net-(U357-DAI) -> Net-(U358-DAO)
- U358 pad 6: Net-(U358-DAI) -> Net-(U357-DAO)
- U359 pad 1: Net-(U358-CLI) -> Net-(U359-CLO)
- U359 pad 3: Net-(U359-CLI) -> Net-(U358-CLO)
- U359 pad 4: Net-(U358-DAI) -> Net-(U359-DAO)
- U359 pad 6: Net-(U359-DAI) -> Net-(U358-DAO)
- U36 pad 1: Net-(U35-CLI) -> Net-(U36-CLO)
- U36 pad 3: Net-(U36-CLI) -> Net-(U35-CLO)
- U36 pad 4: Net-(U35-DAI) -> Net-(U36-DAO)
- U36 pad 6: Net-(U36-DAI) -> Net-(U35-DAO)
- U360 pad 1: Net-(U359-CLI) -> Net-(U360-CLO)
- U360 pad 3: Net-(U360-CLI) -> Net-(U359-CLO)
- U360 pad 4: Net-(U359-DAI) -> Net-(U360-DAO)
- U360 pad 6: Net-(U360-DAI) -> Net-(U359-DAO)
- U361 pad 1: Net-(U360-CLI) -> Net-(U361-CLO)
- U361 pad 3: Net-(U361-CLI) -> Net-(U360-CLO)
- U361 pad 4: Net-(U360-DAI) -> Net-(U361-DAO)
- U361 pad 6: Net-(U361-DAI) -> Net-(U360-DAO)
- U362 pad 1: Net-(U361-CLI) -> Net-(U362-CLO)
- U362 pad 3: Net-(U342-CLO) -> Net-(U361-CLO)
- U362 pad 4: Net-(U361-DAI) -> Net-(U362-DAO)
- U362 pad 6: Net-(U342-DAO) -> Net-(U361-DAO)
- U363 pad 3: Net-(U343-CLO) -> Net-(U362-CLO)
- U363 pad 6: Net-(U343-DAO) -> Net-(U362-DAO)
- U37 pad 1: Net-(U36-CLI) -> Net-(U37-CLO)
- U37 pad 3: Net-(U37-CLI) -> Net-(U36-CLO)
- U37 pad 4: Net-(U36-DAI) -> Net-(U37-DAO)
- U37 pad 6: Net-(U37-DAI) -> Net-(U36-DAO)
- U38 pad 1: Net-(U37-CLI) -> Net-(U38-CLO)
- U38 pad 3: Net-(U38-CLI) -> Net-(U37-CLO)
- U38 pad 4: Net-(U37-DAI) -> Net-(U38-DAO)
- U38 pad 6: Net-(U38-DAI) -> Net-(U37-DAO)
- U383 pad 1: unconnected-(U383-CLO-Pad1) -> Net-(U383-CLO)
- U383 pad 3: Net-(U383-CLI) -> Net-(U382-CLO)
- U383 pad 4: unconnected-(U383-DAO-Pad4) -> Net-(U383-DAO)
- U383 pad 6: Net-(U383-DAI) -> Net-(U382-DAO)
- U384 pad 1: Net-(U383-CLI) -> Net-(U384-CLO)
- U384 pad 3: Net-(U384-CLI) -> Net-(U383-CLO)
- U384 pad 4: Net-(U383-DAI) -> Net-(U384-DAO)
- U384 pad 6: Net-(U384-DAI) -> Net-(U383-DAO)
- U385 pad 1: Net-(U384-CLI) -> Net-(U385-CLO)
- U385 pad 3: Net-(U385-CLI) -> Net-(U384-CLO)
- U385 pad 4: Net-(U384-DAI) -> Net-(U385-DAO)
- U385 pad 6: Net-(U385-DAI) -> Net-(U384-DAO)
- U386 pad 1: Net-(U385-CLI) -> Net-(U386-CLO)
- U386 pad 3: Net-(U386-CLI) -> Net-(U385-CLO)
- U386 pad 4: Net-(U385-DAI) -> Net-(U386-DAO)
- U386 pad 6: Net-(U386-DAI) -> Net-(U385-DAO)
- U387 pad 1: Net-(U386-CLI) -> Net-(U387-CLO)
- U387 pad 3: Net-(U387-CLI) -> Net-(U386-CLO)
- U387 pad 4: Net-(U386-DAI) -> Net-(U387-DAO)
- U387 pad 6: Net-(U387-DAI) -> Net-(U386-DAO)
- U388 pad 1: Net-(U387-CLI) -> Net-(U388-CLO)
- U388 pad 3: Net-(U388-CLI) -> Net-(U387-CLO)
- U388 pad 4: Net-(U387-DAI) -> Net-(U388-DAO)
- U388 pad 6: Net-(U388-DAI) -> Net-(U387-DAO)
- U389 pad 1: Net-(U388-CLI) -> Net-(U389-CLO)
- U389 pad 3: Net-(U389-CLI) -> Net-(U388-CLO)
- U389 pad 4: Net-(U388-DAI) -> Net-(U389-DAO)
- U389 pad 6: Net-(U389-DAI) -> Net-(U388-DAO)
- U39 pad 1: Net-(U38-CLI) -> Net-(U39-CLO)
- U39 pad 3: Net-(U39-CLI) -> Net-(U38-CLO)
- U39 pad 4: Net-(U38-DAI) -> Net-(U39-DAO)
- U39 pad 6: Net-(U39-DAI) -> Net-(U38-DAO)
- U390 pad 1: Net-(U389-CLI) -> Net-(U390-CLO)
- U390 pad 3: Net-(U390-CLI) -> Net-(U389-CLO)
- U390 pad 4: Net-(U389-DAI) -> Net-(U390-DAO)
- U390 pad 6: Net-(U390-DAI) -> Net-(U389-DAO)
- U391 pad 1: Net-(U390-CLI) -> Net-(U391-CLO)
- U391 pad 3: Net-(U391-CLI) -> Net-(U390-CLO)
- U391 pad 4: Net-(U390-DAI) -> Net-(U391-DAO)
- U391 pad 6: Net-(U391-DAI) -> Net-(U390-DAO)
- U392 pad 1: Net-(U391-CLI) -> Net-(U392-CLO)
- U392 pad 3: Net-(U392-CLI) -> Net-(U391-CLO)
- U392 pad 4: Net-(U391-DAI) -> Net-(U392-DAO)
- U392 pad 6: Net-(U392-DAI) -> Net-(U391-DAO)
- U393 pad 1: Net-(U392-CLI) -> Net-(U393-CLO)
- U393 pad 3: Net-(U393-CLI) -> Net-(U392-CLO)
- U393 pad 4: Net-(U392-DAI) -> Net-(U393-DAO)
- U393 pad 6: Net-(U393-DAI) -> Net-(U392-DAO)
- U394 pad 1: Net-(U393-CLI) -> Net-(U394-CLO)
- U394 pad 3: Net-(U394-CLI) -> Net-(U393-CLO)
- U394 pad 4: Net-(U393-DAI) -> Net-(U394-DAO)
- U394 pad 6: Net-(U394-DAI) -> Net-(U393-DAO)
- U395 pad 1: Net-(U394-CLI) -> Net-(U395-CLO)
- U395 pad 3: Net-(U395-CLI) -> Net-(U394-CLO)
- U395 pad 4: Net-(U394-DAI) -> Net-(U395-DAO)
- U395 pad 6: Net-(U395-DAI) -> Net-(U394-DAO)
- U396 pad 1: Net-(U395-CLI) -> Net-(U396-CLO)
- U396 pad 3: Net-(U396-CLI) -> Net-(U395-CLO)
- U396 pad 4: Net-(U395-DAI) -> Net-(U396-DAO)
- U396 pad 6: Net-(U396-DAI) -> Net-(U395-DAO)
- U397 pad 1: Net-(U396-CLI) -> Net-(U397-CLO)
- U397 pad 3: Net-(U397-CLI) -> Net-(U396-CLO)
- U397 pad 4: Net-(U396-DAI) -> Net-(U397-DAO)
- U397 pad 6: Net-(U397-DAI) -> Net-(U396-DAO)
- U398 pad 1: Net-(U397-CLI) -> Net-(U398-CLO)
- U398 pad 3: Net-(U398-CLI) -> Net-(U397-CLO)
- U398 pad 4: Net-(U397-DAI) -> Net-(U398-DAO)
- U398 pad 6: Net-(U398-DAI) -> Net-(U397-DAO)
- U399 pad 1: Net-(U398-CLI) -> Net-(U399-CLO)
- U399 pad 3: Net-(U399-CLI) -> Net-(U398-CLO)
- U399 pad 4: Net-(U398-DAI) -> Net-(U399-DAO)
- U399 pad 6: Net-(U399-DAI) -> Net-(U398-DAO)
- U40 pad 1: Net-(U39-CLI) -> Net-(U40-CLO)
- U40 pad 3: Net-(U40-CLI) -> Net-(U39-CLO)
- U40 pad 4: Net-(U39-DAI) -> Net-(U40-DAO)
- U40 pad 6: Net-(U40-DAI) -> Net-(U39-DAO)
- U400 pad 1: Net-(U399-CLI) -> Net-(U400-CLO)
- U400 pad 3: Net-(U400-CLI) -> Net-(U399-CLO)
- U400 pad 4: Net-(U399-DAI) -> Net-(U400-DAO)
- U400 pad 6: Net-(U400-DAI) -> Net-(U399-DAO)
- U401 pad 1: Net-(U400-CLI) -> Net-(U401-CLO)
- U401 pad 3: Net-(U401-CLI) -> Net-(U400-CLO)
- U401 pad 4: Net-(U400-DAI) -> Net-(U401-DAO)
- U401 pad 6: Net-(U401-DAI) -> Net-(U400-DAO)
- U402 pad 1: Net-(U401-CLI) -> unconnected-(U402-CLO-Pad1)
- U402 pad 3: Net-(U382-CLO) -> Net-(U401-CLO)
- U402 pad 4: Net-(U401-DAI) -> unconnected-(U402-DAO-Pad4)
- U402 pad 6: Net-(U382-DAO) -> Net-(U401-DAO)
- U41 pad 1: Net-(U40-CLI) -> Net-(U41-CLO)
- U41 pad 3: Net-(U41-CLI) -> Net-(U40-CLO)
- U41 pad 4: Net-(U40-DAI) -> Net-(U41-DAO)
- U41 pad 6: Net-(U41-DAI) -> Net-(U40-DAO)
- U42 pad 1: Net-(U41-CLI) -> Net-(U42-CLO)
- U42 pad 3: Net-(U22-CLO) -> Net-(U41-CLO)
- U42 pad 4: Net-(U41-DAI) -> Net-(U42-DAO)
- U42 pad 6: Net-(U22-DAO) -> Net-(U41-DAO)
- U43 pad 3: Net-(U23-CLO) -> Net-(U42-CLO)
- U43 pad 6: Net-(U23-DAO) -> Net-(U42-DAO)
- U63 pad 3: Net-(U63-CLI) -> Net-(U62-CLO)
- U63 pad 6: Net-(U63-DAI) -> Net-(U62-DAO)
- U64 pad 1: Net-(U63-CLI) -> Net-(U64-CLO)
- U64 pad 3: Net-(U64-CLI) -> Net-(U63-CLO)
- U64 pad 4: Net-(U63-DAI) -> Net-(U64-DAO)
- U64 pad 6: Net-(U64-DAI) -> Net-(U63-DAO)
- U65 pad 1: Net-(U64-CLI) -> Net-(U65-CLO)
- U65 pad 3: Net-(U65-CLI) -> Net-(U64-CLO)
- U65 pad 4: Net-(U64-DAI) -> Net-(U65-DAO)
- U65 pad 6: Net-(U65-DAI) -> Net-(U64-DAO)
- U66 pad 1: Net-(U65-CLI) -> Net-(U66-CLO)
- U66 pad 3: Net-(U66-CLI) -> Net-(U65-CLO)
- U66 pad 4: Net-(U65-DAI) -> Net-(U66-DAO)
- U66 pad 6: Net-(U66-DAI) -> Net-(U65-DAO)
- U67 pad 1: Net-(U66-CLI) -> Net-(U67-CLO)
- U67 pad 3: Net-(U67-CLI) -> Net-(U66-CLO)
- U67 pad 4: Net-(U66-DAI) -> Net-(U67-DAO)
- U67 pad 6: Net-(U67-DAI) -> Net-(U66-DAO)
- U68 pad 1: Net-(U67-CLI) -> Net-(U68-CLO)
- U68 pad 3: Net-(U68-CLI) -> Net-(U67-CLO)
- U68 pad 4: Net-(U67-DAI) -> Net-(U68-DAO)
- U68 pad 6: Net-(U68-DAI) -> Net-(U67-DAO)
- U69 pad 1: Net-(U68-CLI) -> Net-(U69-CLO)
- U69 pad 3: Net-(U69-CLI) -> Net-(U68-CLO)
- U69 pad 4: Net-(U68-DAI) -> Net-(U69-DAO)
- U69 pad 6: Net-(U69-DAI) -> Net-(U68-DAO)
- U70 pad 1: Net-(U69-CLI) -> Net-(U70-CLO)
- U70 pad 3: Net-(U70-CLI) -> Net-(U69-CLO)
- U70 pad 4: Net-(U69-DAI) -> Net-(U70-DAO)
- U70 pad 6: Net-(U70-DAI) -> Net-(U69-DAO)
- U71 pad 1: Net-(U70-CLI) -> Net-(U71-CLO)
- U71 pad 3: Net-(U71-CLI) -> Net-(U70-CLO)
- U71 pad 4: Net-(U70-DAI) -> Net-(U71-DAO)
- U71 pad 6: Net-(U71-DAI) -> Net-(U70-DAO)
- U72 pad 1: Net-(U71-CLI) -> Net-(U72-CLO)
- U72 pad 3: Net-(U72-CLI) -> Net-(U71-CLO)
- U72 pad 4: Net-(U71-DAI) -> Net-(U72-DAO)
- U72 pad 6: Net-(U72-DAI) -> Net-(U71-DAO)
- U73 pad 1: Net-(U72-CLI) -> Net-(U73-CLO)
- U73 pad 3: Net-(U73-CLI) -> Net-(U72-CLO)
- U73 pad 4: Net-(U72-DAI) -> Net-(U73-DAO)
- U73 pad 6: Net-(U73-DAI) -> Net-(U72-DAO)
- U74 pad 1: Net-(U73-CLI) -> Net-(U74-CLO)
- U74 pad 3: Net-(U74-CLI) -> Net-(U73-CLO)
- U74 pad 4: Net-(U73-DAI) -> Net-(U74-DAO)
- U74 pad 6: Net-(U74-DAI) -> Net-(U73-DAO)
- U75 pad 1: Net-(U74-CLI) -> Net-(U75-CLO)
- U75 pad 3: Net-(U75-CLI) -> Net-(U74-CLO)
- U75 pad 4: Net-(U74-DAI) -> Net-(U75-DAO)
- U75 pad 6: Net-(U75-DAI) -> Net-(U74-DAO)
- U76 pad 1: Net-(U75-CLI) -> Net-(U76-CLO)
- U76 pad 3: Net-(U76-CLI) -> Net-(U75-CLO)
- U76 pad 4: Net-(U75-DAI) -> Net-(U76-DAO)
- U76 pad 6: Net-(U76-DAI) -> Net-(U75-DAO)
- U77 pad 1: Net-(U76-CLI) -> Net-(U77-CLO)
- U77 pad 3: Net-(U77-CLI) -> Net-(U76-CLO)
- U77 pad 4: Net-(U76-DAI) -> Net-(U77-DAO)
- U77 pad 6: Net-(U77-DAI) -> Net-(U76-DAO)
- U78 pad 1: Net-(U77-CLI) -> Net-(U78-CLO)
- U78 pad 3: Net-(U78-CLI) -> Net-(U77-CLO)
- U78 pad 4: Net-(U77-DAI) -> Net-(U78-DAO)
- U78 pad 6: Net-(U78-DAI) -> Net-(U77-DAO)
- U79 pad 1: Net-(U78-CLI) -> Net-(U79-CLO)
- U79 pad 3: Net-(U79-CLI) -> Net-(U78-CLO)
- U79 pad 4: Net-(U78-DAI) -> Net-(U79-DAO)
- U79 pad 6: Net-(U79-DAI) -> Net-(U78-DAO)
- U80 pad 1: Net-(U79-CLI) -> Net-(U80-CLO)
- U80 pad 3: Net-(U80-CLI) -> Net-(U79-CLO)
- U80 pad 4: Net-(U79-DAI) -> Net-(U80-DAO)
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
